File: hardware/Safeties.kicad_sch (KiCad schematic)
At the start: 12 parts, among them K1 ALDP105W, Q1 2N7002, Q2 2N7002, U14 74AUP1G32

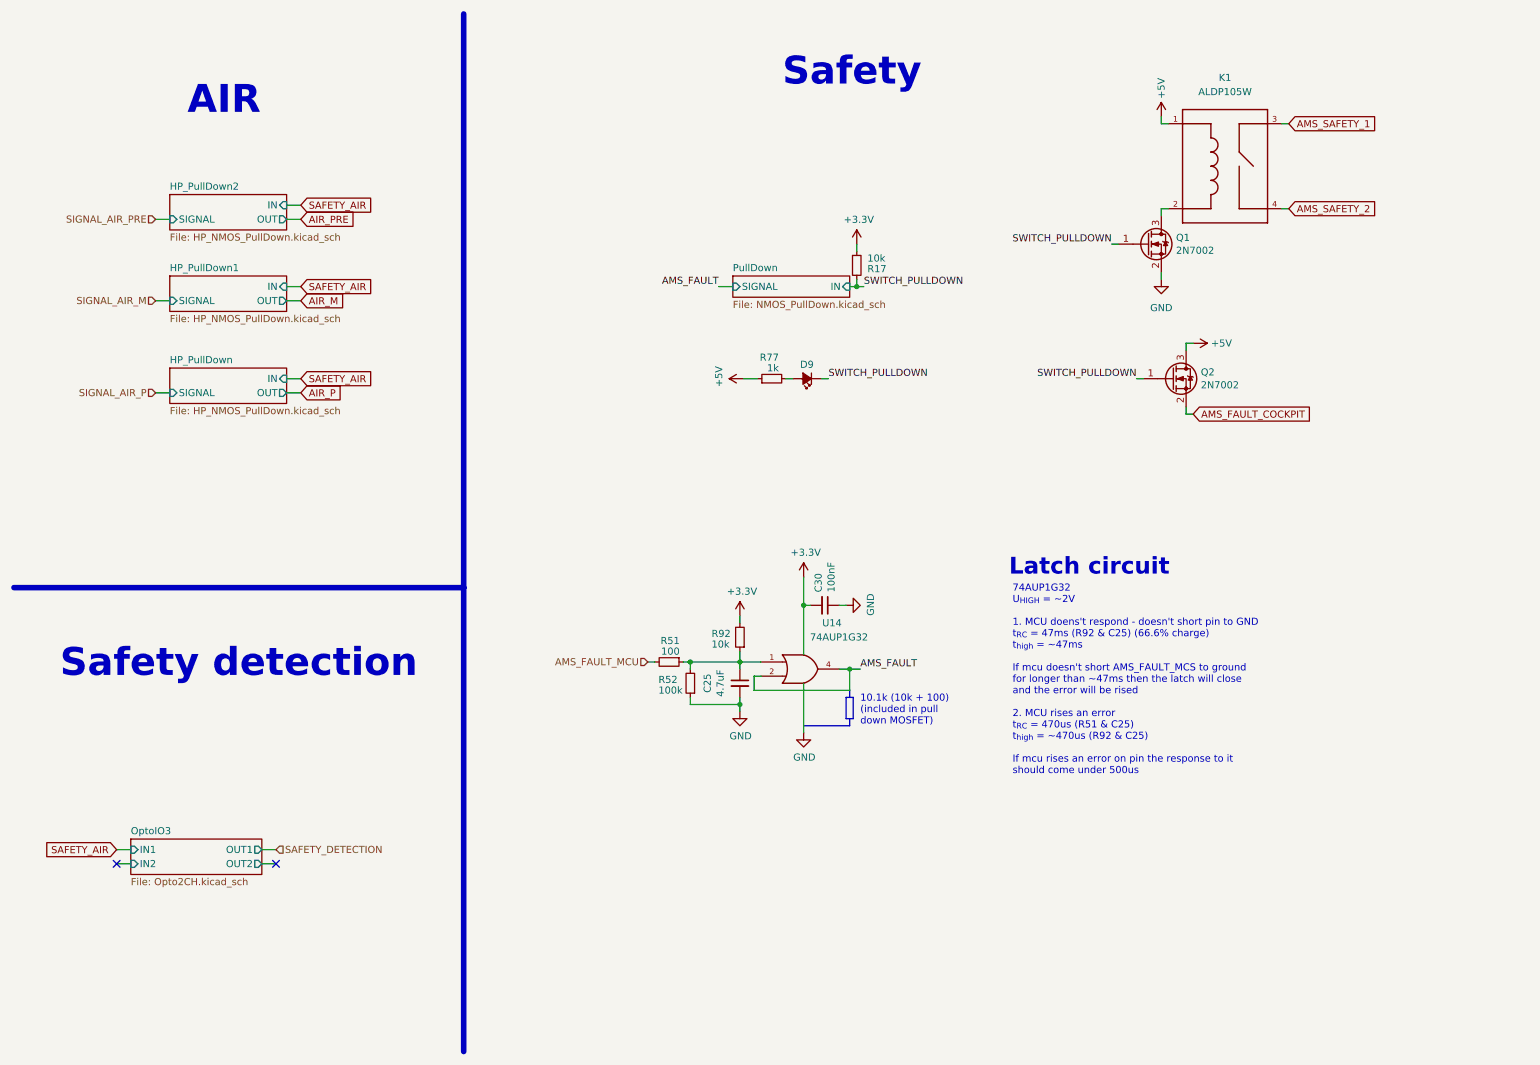
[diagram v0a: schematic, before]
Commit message: schemat sync
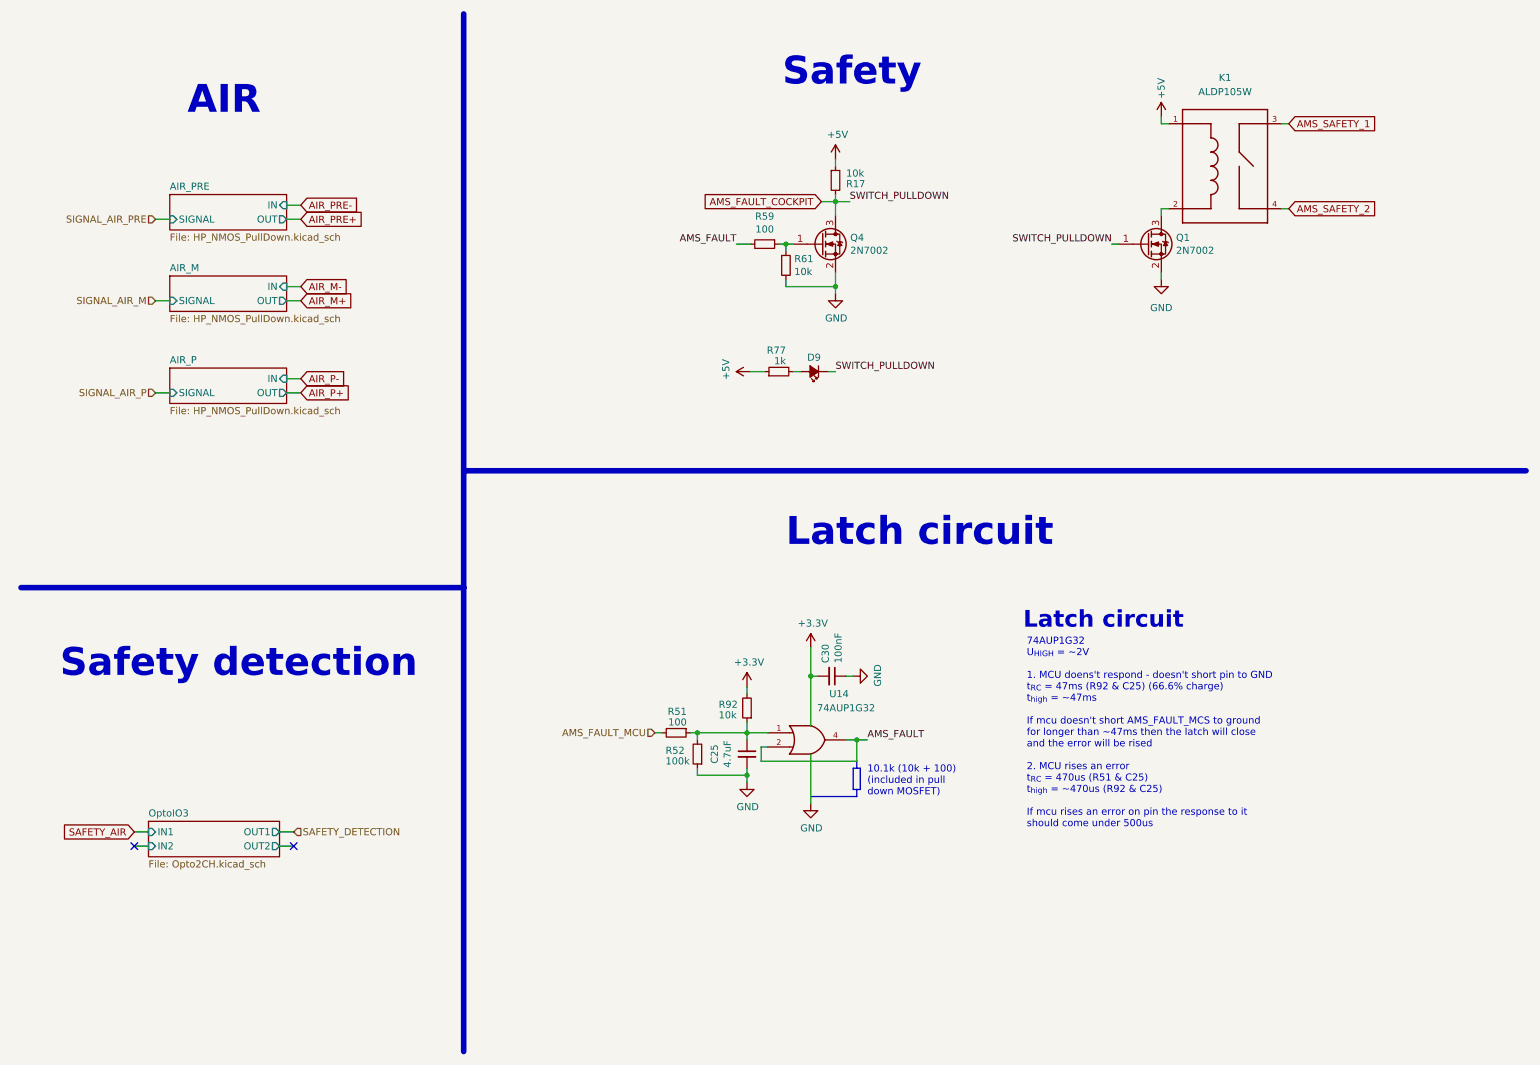
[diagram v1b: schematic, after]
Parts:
- removed Q2: 2N7002, Package_TO_SOT_SMD:SOT-23, symbol Transistor_FET:2N7002
- added Q4: 2N7002, Package_TO_SOT_SMD:SOT-23, symbol Transistor_FET:2N7002
- added R59: 100, Resistor_SMD:R_0603_1608Metric, symbol Device:R_Small
- added R61: 10k, Resistor_SMD:R_0603_1608Metric, symbol Device:R_Small
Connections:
- net SWITCH_PULLDOWN is gone; now on net AMS_FAULT_COCKPIT: D9.1 (K), Q1.1 (G), R17.2
- net +3V3: no longer R17.1
- net +5V: now also R17.1
- net AMS_FAULT: now also R59.2
- net AMS_FAULT_COCKPIT: now also Q4.3 (D)
- net GND: now also Q4.2 (S), R61.2
- new net: Q4.1 (G), R59.1, R61.1
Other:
- sheet HP_PullDown renamed AIR_P
- sheet HP_PullDown1 renamed AIR_M
- sheet HP_PullDown2 renamed AIR_PRE
- removed sheet PullDown
- moved on the sheet: C25, C30, D9, R17, R51, R52, R77, R92, U14
